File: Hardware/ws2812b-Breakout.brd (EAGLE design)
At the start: 17.8 x 12.7 mm, 11 parts, among them U1 WS2812B

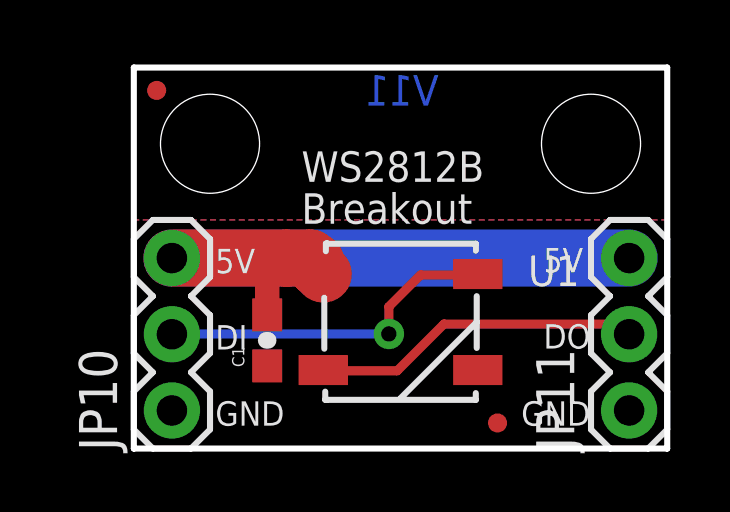
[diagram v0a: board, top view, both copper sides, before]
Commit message: Fixed qc issues
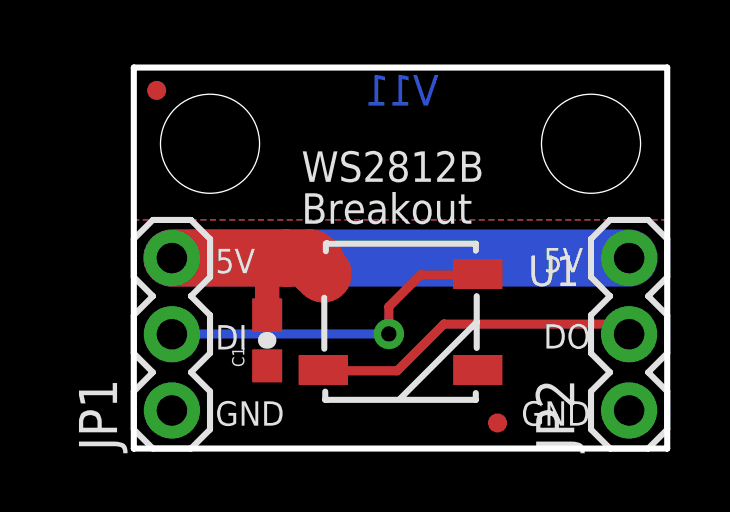
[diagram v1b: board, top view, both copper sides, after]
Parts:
- removed JP10: INPUT, SparkFun-Connectors:1X03
- added JP15: STAND-OFF, SparkFun:STAND-OFF
- JP1: value STAND-OFF -> INPUT; device SparkFun:STAND-OFF -> SparkFun-Connectors:1X03
- moved JP1 16.6 mm to (1.27, 1.27), turned to 90 degrees
- renumbered JP11 to JP2
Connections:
- net DI: now also JP1.2; no longer JP10.2
- net GND: now also JP1.1; no longer JP10.1
- net VCC: now also JP1.3; no longer JP10.3
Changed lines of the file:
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@@
 <attribute name="VALUE" value="0.1uF" x="4.445" y="3.6068" size="1.778" layer="27" rot="R90" display="off"/>
 </element>
-<element name="JP1" library="SparkFun" package="STAND-OFF" value="STAND-OFF" x="15.24" y="10.16"/>
+<element name="JP15" library="SparkFun" package="STAND-OFF" value="STAND-OFF" x="15.24" y="10.16"/>
 <element name="JP4" library="SparkFun" package="STAND-OFF" value="STAND-OFF" x="2.54" y="10.16"/>
-<element name="JP10" library="SparkFun-Connectors" package="1X03" value="INPUT" x="1.27" y="1.27" rot="R90"/>
-<element name="JP11" library="SparkFun-Connectors" package="1X03" value="OUTPUT" x="16.51" y="1.27" rot="R90"/>
+<element name="JP1" library="SparkFun-Connectors" package="1X03" value="INPUT" x="1.27" y="1.27" rot="R90"/>
+<element name="JP2" library="SparkFun-Connectors" package="1X03" value="OUTPUT" x="16.51" y="1.27" rot="R90"/>
 <element name="LOGO1" library="SparkFun-Aesthetics" package="OSHW-LOGO-S" value="OSHW-LOGOS" x="8.976359375" y="9.136378125" rot="MR0"/>
 <element name="FID1" library="SparkFun-Aesthetics" package="MICRO-FIDUCIAL" value="FIDUCIALUFIDUCIAL" x="0.762" y="11.938"/>
@@
 <signal name="VCC">
 <contactref element="C1" pad="2"/>
-<contactref element="JP10" pad="3"/>
-<contactref element="JP11" pad="3"/>
+<contactref element="JP1" pad="3"/>
+<contactref element="JP2" pad="3"/>
 <wire x1="16.51" y1="6.35" x2="1.27" y2="6.35" width="1.905" layer="16"/>
 <contactref element="U1" pad="1"/>
@@
 <vertex x="17.78" y="7.62"/>
 </polygon>
-<contactref element="JP10" pad="1"/>
-<contactref element="JP11" pad="1"/>
+<contactref element="JP1" pad="1"/>
+<contactref element="JP2" pad="1"/>
 <contactref element="U1" pad="3"/>
 </signal>
 <signal name="DO">
-<contactref element="JP11" pad="2"/>
+<contactref element="JP2" pad="2"/>
 <contactref element="U1" pad="2"/>
 <wire x1="8.778440625" y1="2.591" x2="10.3378" y2="4.150359375" width="0.3048" layer="1"/>
@@
 </signal>
 <signal name="DI">
-<contactref element="JP10" pad="2"/>
+<contactref element="JP1" pad="2"/>
 <via x="8.50138125" y="3.820159375" extent="1-16" drill="0.508"/>
 <contactref element="U1" pad="4"/>
